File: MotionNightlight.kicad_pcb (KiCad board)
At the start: 2 copper layers, 72 x 42 mm, 9 parts, among them J1 Conn_02x04_Odd_Even, M2 MountingHole_2.2mm_M2_Pad_Via, Q1 IRL3803

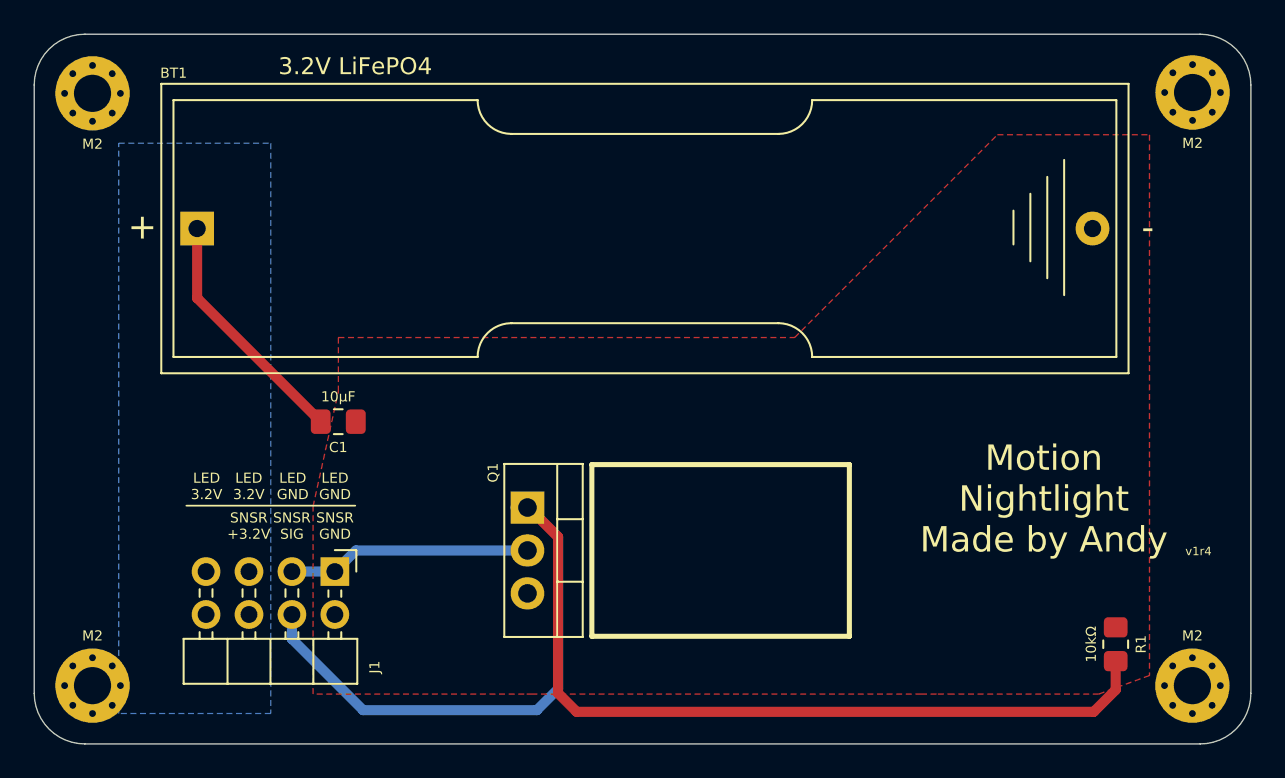
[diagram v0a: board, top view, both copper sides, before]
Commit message: v2r1
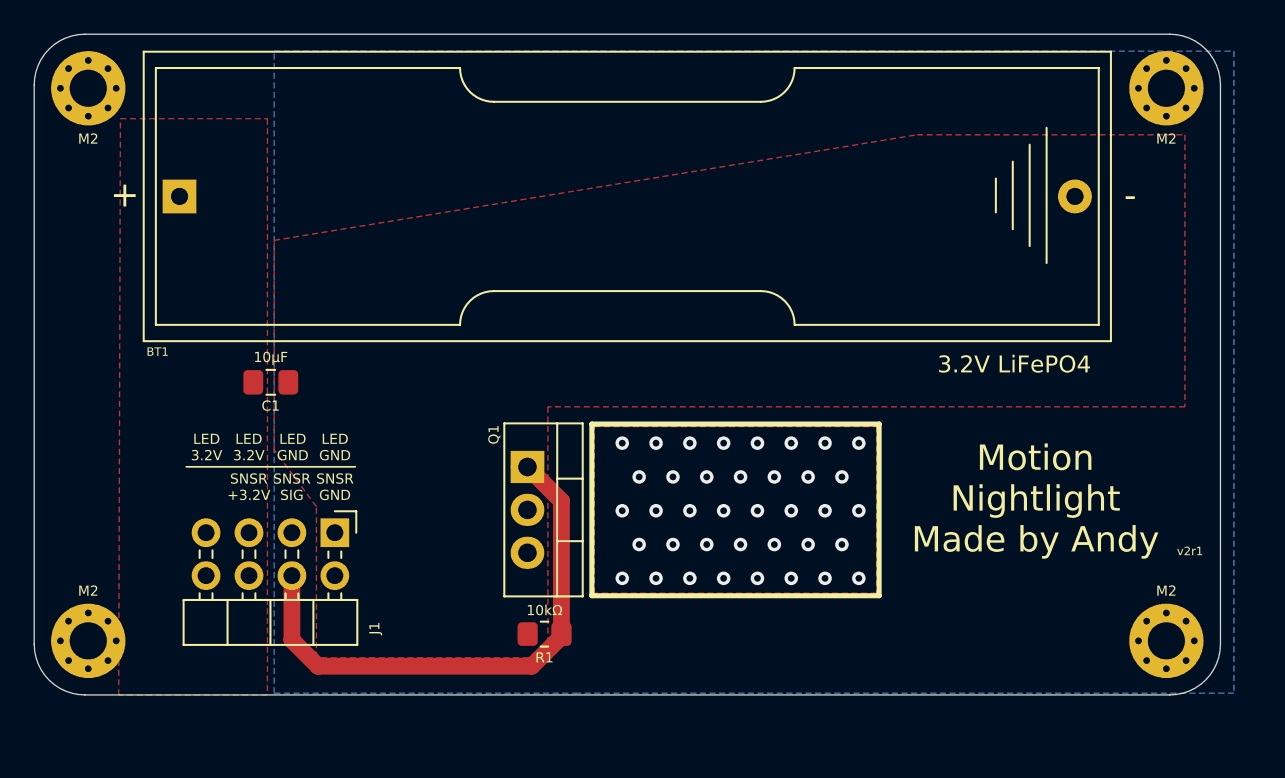
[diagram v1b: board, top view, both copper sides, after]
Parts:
- moved R1 33.8 mm to (125.2, 85.5), turned to 0 degrees
- moved C1 4.62 mm to (109.0, 70.6)
- moved M2 3.06 mm to (162.0, 85.9)
- moved M2 2.66 mm to (98.2, 85.9)
- moved Q1 2.40 mm to (124.2, 75.6)
- moved J1 2.30 mm to (112.8, 79.5)
- moved BT1 2.17 mm to (104.1, 59.6)
- moved M2 1.57 mm to (162.0, 53.2)
- moved M2 0.39 mm to (98.2, 53.2)
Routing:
- net /FET-GATE: track 80.6 -> 34.1 mm
- net /+3.2V: track 14.5 -> 0.00 mm
- net /FET-DRN: track 14.5 -> 0.00 mm, vias 0 -> 38
- added copper zone on F.Cu, net /+3.2V
- added copper zone on B.Cu, net /FET-DRN
- added copper zone on F.Cu, net /FET-DRN
- removed copper zone on B.Cu, net /+3.2V
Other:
- board size 72 x 42 mm -> 70.2 x 39.1 mm
- board text added: "v2r1"
- board text removed: "v1r4"
